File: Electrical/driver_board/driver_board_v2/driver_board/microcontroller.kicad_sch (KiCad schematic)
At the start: 24 parts, among them J1 USB_C_Receptacle_USB2.0_14P, J2 Conn_01x04_Pin, SW1 SW_SPDT, SW2 SW_Push, U1 STM32F446RETx, Y1 8Mhz

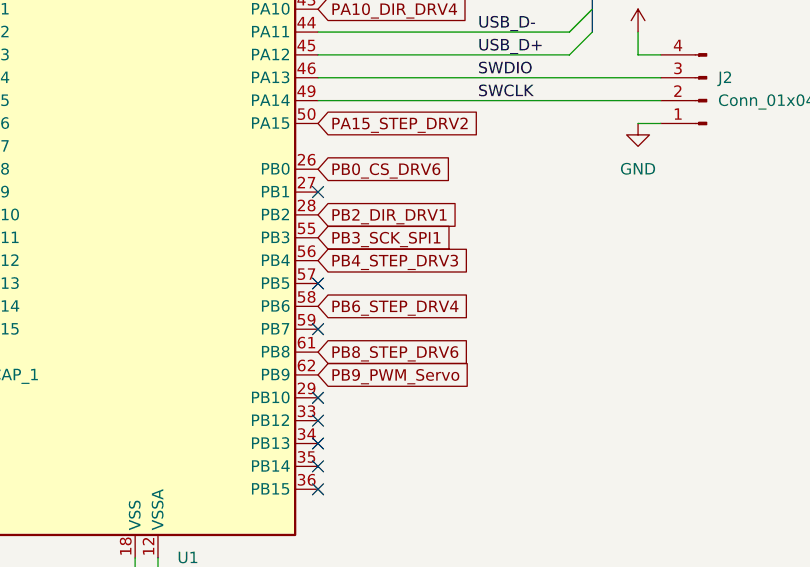
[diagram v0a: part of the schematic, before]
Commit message: Finished TMC Labeling
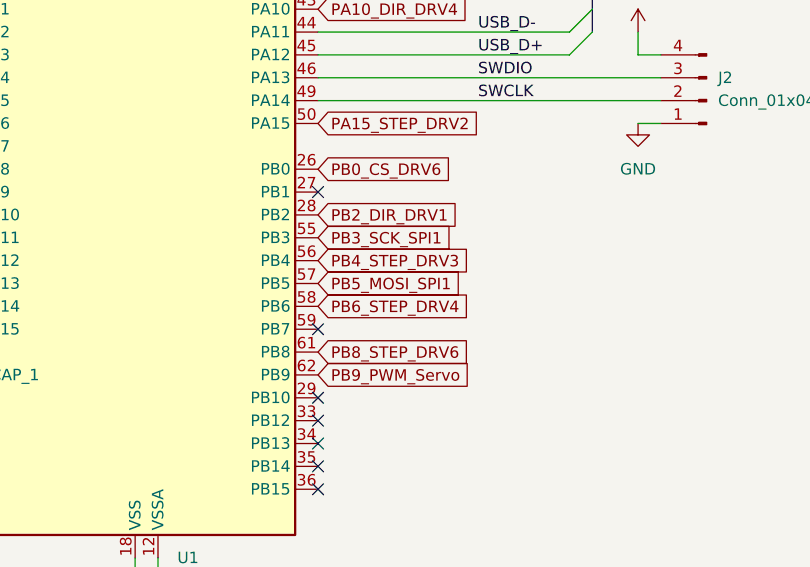
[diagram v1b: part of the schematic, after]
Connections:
- net PB5_MOSI_SPI1: now reaches U1.57 (PB5)
- no-connect marks 23 -> 22
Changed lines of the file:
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@@
-	)
-	(no_connect
-		(at 147.32 119.38)
 	)
 	(no_connect
@@
 			(effects
 				(font
+					(size 1.27 1.27)
+				)
+				(justify left)
+				(hide yes)
+			)
+		)
+	)
+	(global_label "PB5_MOSI_SPI1"
+		(shape input)
+		(at 147.32 119.38 0)
+		(fields_autoplaced yes)
+		(effects
+			(font
+				(size 1.27 1.27)
+			)
+			(justify left)
+		)
+		(property "Intersheetrefs" "${INTERSHEET_REFS}"
+			(at 164.8799 119.38 0)
+			(effects
+				(font
